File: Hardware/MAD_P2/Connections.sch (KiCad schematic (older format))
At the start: 48 parts, among them J10 Conn_02x05_Odd_Even, J11 Conn_02x05_Odd_Even, J13 Conn_02x05_Odd_Even, J14 Conn_02x05_Odd_Even, J15 Conn_ADC1, J16 Conn_DAC, J18 P3, J19 P4, J20 P2, J21 Conn_02x05_Odd_Even, J22 Conn_02x05_Odd_Even, J23 Conn_02x03_Odd_Even, J24 P5, J25 P6, J26 P7, J31 Micro_SD_Card_Connector, J32 Micro_SD_Card_Socket, J6 Edge_Conn, J7 Conn_02x05_Odd_Even, J8 USB_C_Receptacle_USB2.0, J9 Conn_02x05_Odd_Even, Q1 MMBT3904, U27 FT232RL

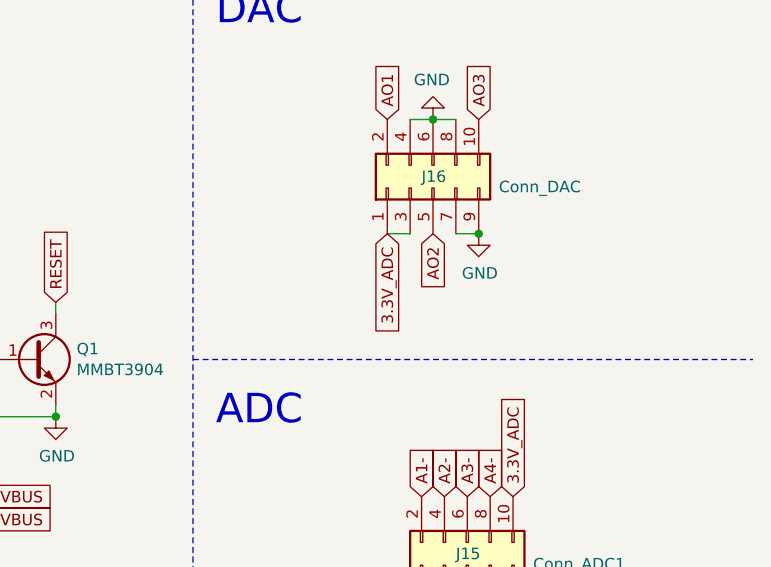
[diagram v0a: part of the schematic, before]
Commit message: test
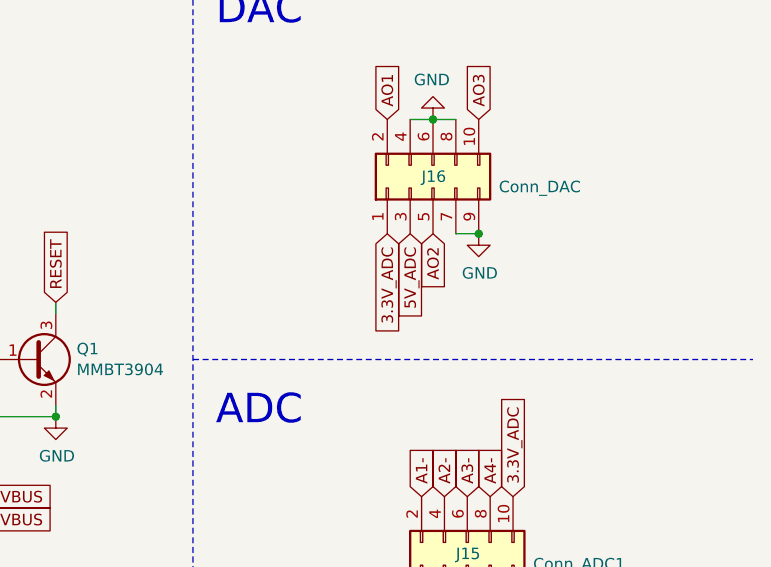
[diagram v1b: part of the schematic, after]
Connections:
- net 3.3V_ADC: no longer J16.3 (Pin_3)
- new net 5V_ADC: J16.3 (Pin_3)
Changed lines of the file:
@@
 $EndComp
-Wire Wire Line
-	9600 1650 9700 1650
 Wire Wire Line
 	9900 1650 10000 1650
@@
 Text GLabel 6200 6100 0    50   Input ~ 0
 P39
+Text GLabel 9700 1650 3    50   Input ~ 0
+5V_ADC
 $EndSCHEMATC
